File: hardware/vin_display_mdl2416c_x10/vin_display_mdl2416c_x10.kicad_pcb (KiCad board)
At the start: 2 copper layers, 176.7 x 50.9 mm, 62 parts, among them J1 DEBUG, J2 USB_B_Micro, J3 DEBUG_UART, J4 Conn_01x04, J5 AUX_CONNECTOR, Q1 BSS138, SW1 SW_RESET, SW2 BOOTSEL, SW3 KNOB, U1 W25Q16JVSNIQ, U10 MDL2416C, U11 MDL2416C, U12 MDL2416C, U13 MDL2416C, U14 MDL2416C, U2 MIC23050-SYML, U3 RP2040, U4 HEF4028BT, U5 MDL2416C, U6 MDL2416C, U7 MDL2416C, U8 MDL2416C, U9 MDL2416C, X1 12MHz

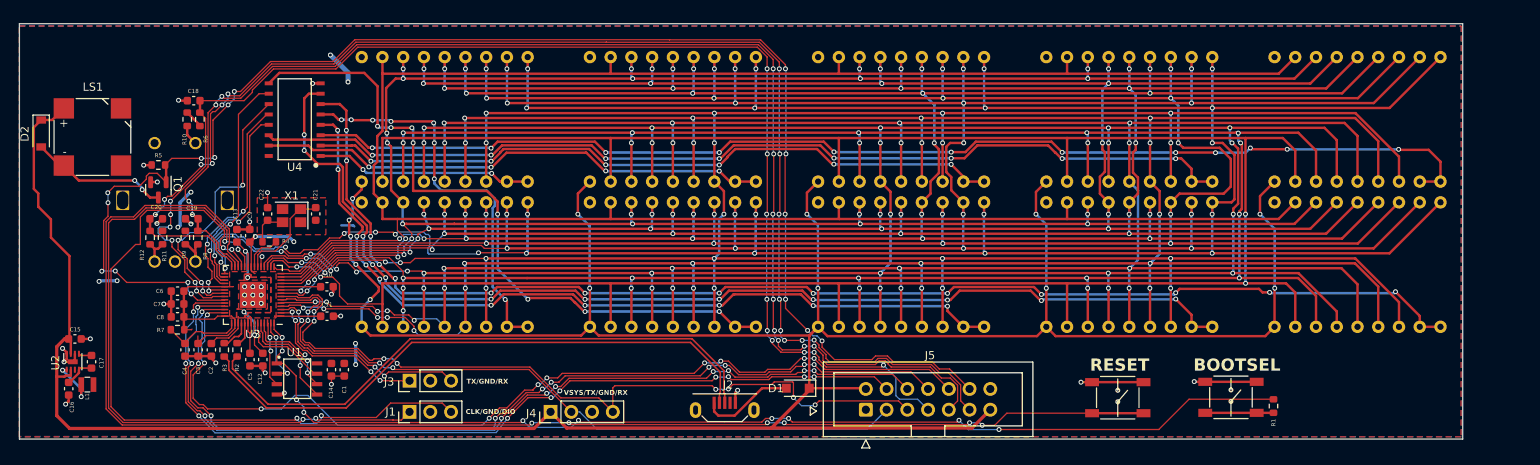
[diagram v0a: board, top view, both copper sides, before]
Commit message: minor schematic fixes
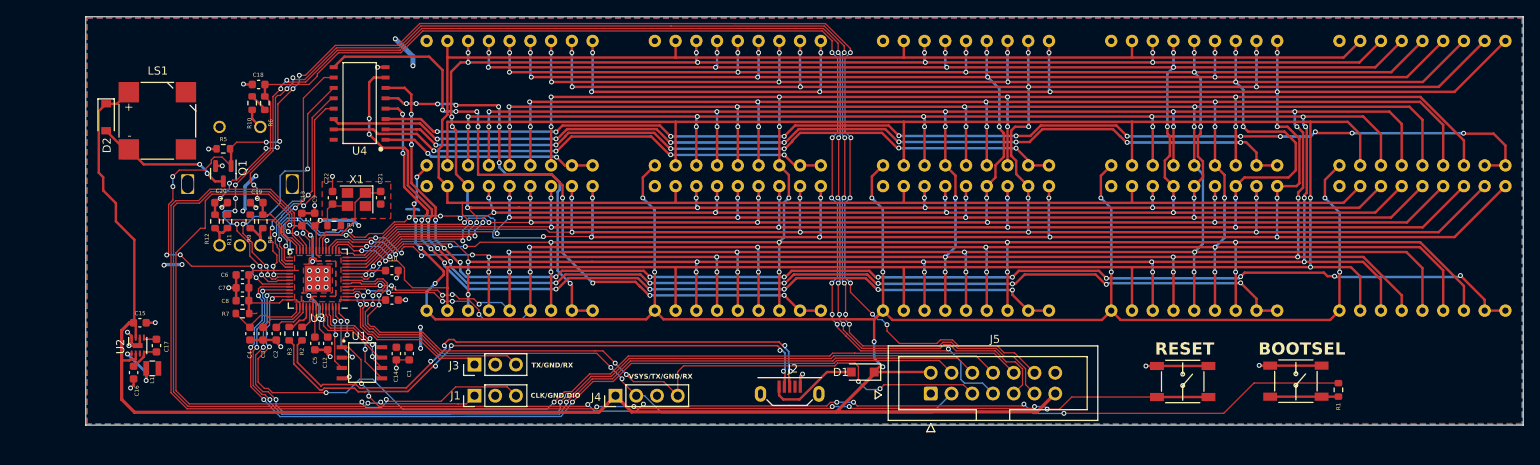
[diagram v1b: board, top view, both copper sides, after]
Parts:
- C21, C22: value 15p -> 19p
- J4: value Conn_01x04 -> IF_UART
- moved C1 8.19 mm to (106.6, 116.7)
- moved C10 8.19 mm to (104.5, 106.6)
- moved C11 8.19 mm to (104.5, 110.2)
- moved C12 8.19 mm to (96.6, 115.5)
- moved C13 8.19 mm to (93.5, 100.3)
- moved C17 8.19 mm to (75.7, 115.8)
- moved C2 8.19 mm to (90.3, 114.3)
- moved C20 8.19 mm to (83.6, 98.3)
- moved C21 8.19 mm to (103.1, 97.7)
- moved C5 8.19 mm to (95.1, 115.5)
- moved C7 8.19 mm to (86.2, 108.7)
- moved J4 8.19 mm to (131.9, 121.9)
- moved R10 8.19 mm to (87.4, 86.1)
- moved R12 8.19 mm to (82.8, 100.6)
- moved R4 8.19 mm to (97.4, 101.1)
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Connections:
- SW3 pad G: GND -> (no net)
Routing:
- net GP29: track 114.8 -> 112.6 mm, vias 10 -> 4
- net GP28: track 112.7 -> 110.6 mm, vias 10 -> 4
- net GP27: track 110.4 -> 109.2 mm, vias 10 -> 4
- net USB_DP: track 72.6 -> 73.8 mm, vias 0 -> 4
- net VSYS: track 398.1 -> 399.2 mm, vias 13 -> 15
- net SPEAKER: track 182.3 -> 183.4 mm
- net KNOB_SW: track 165.3 -> 166.3 mm, vias 15 -> 13
- net 3V3: track 72.7 -> 71.8 mm
- net USB_DN: track 72.6 -> 73.1 mm, vias 0 -> 4
- net ENC_B: track 168.5 -> 168.9 mm, vias 14 -> 12
- net UART0_RX: track 27.7 -> 27.2 mm, vias 4 -> 2
- net ENC_A: track 161.0 -> 160.5 mm, vias 12 -> 10
- net UART1_RX: track 95.9 -> 95.7 mm, vias 8 -> 6
- net GP26: track 107.5 -> 107.6 mm, vias 10 -> 4
- net UART0_TX: vias 4 -> 2
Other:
- board size 176.7 x 50.9 mm -> 176 x 50 mm
